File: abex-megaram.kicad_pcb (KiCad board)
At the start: 2 copper layers, 135.5 x 71.5 mm, 56 parts, among them P1 0877159106, P2 CONN_01X01, P3 CONN_01X01, P4 CONN_01X01, P5 CONN_01X01, P6 CONN_01X01, SW1 SW_DIP_x03, SW2 SW_Push, U1 74HC04, U14 STM32F407VGTx, U7 ISSI61WV5128BL, U8 ISSI61WV5128BL

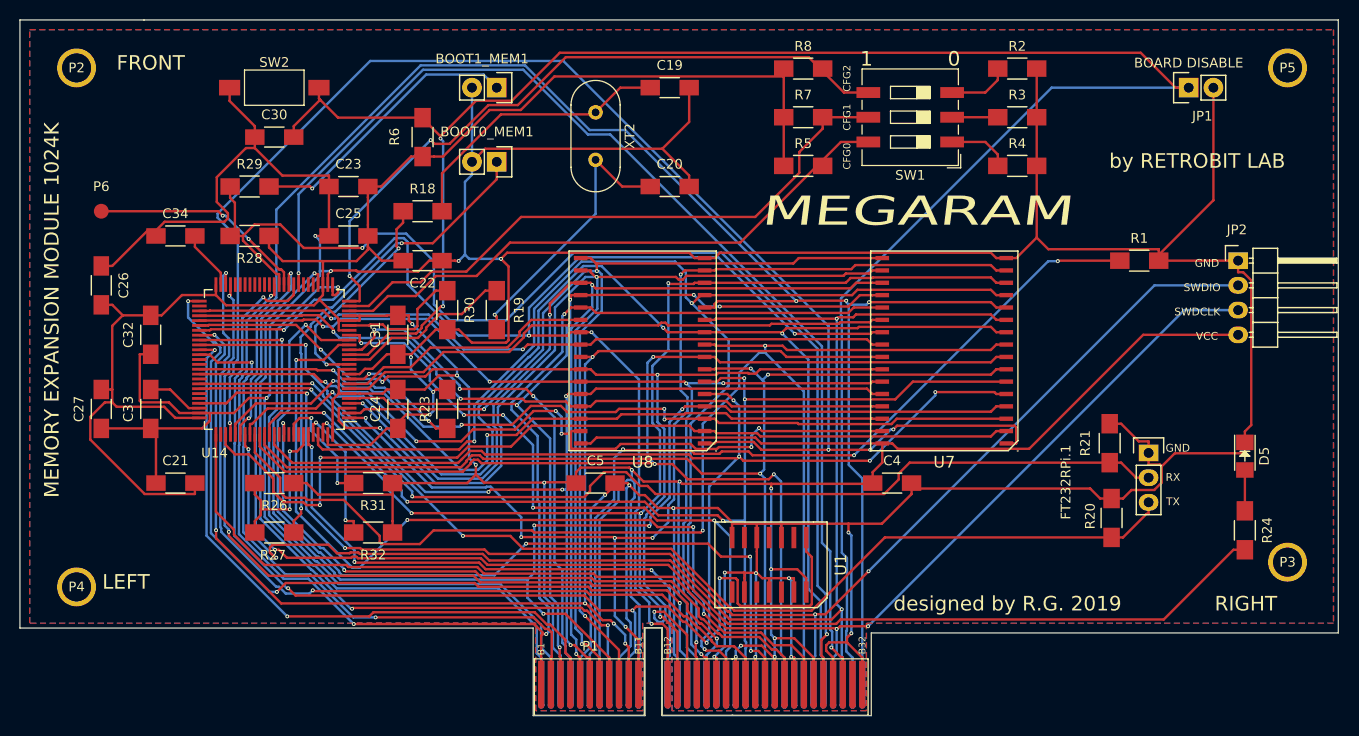
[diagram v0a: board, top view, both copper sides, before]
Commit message: New layout and design
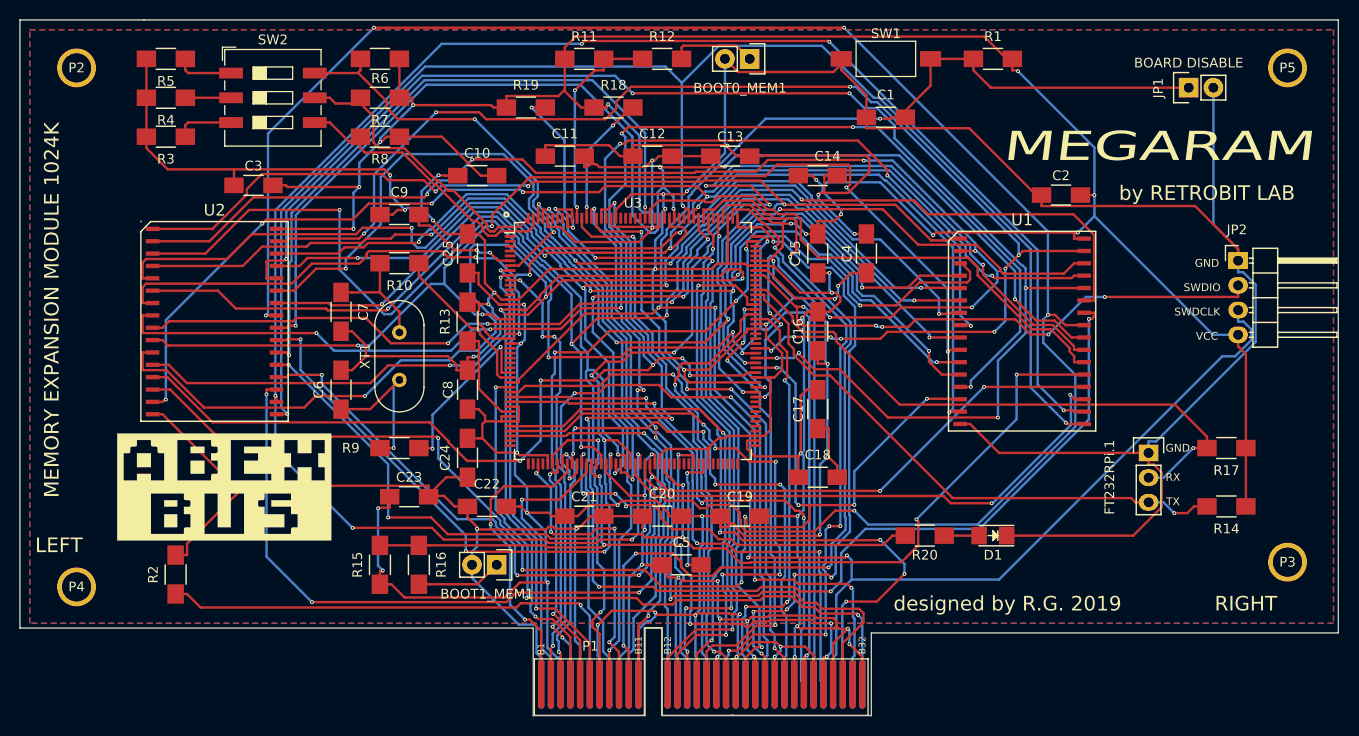
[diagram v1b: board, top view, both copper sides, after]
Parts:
- removed C26, C27, C30, C31: 100n, Capacitors_SMD:C_1206_HandSoldering
- removed C32: 1u, Capacitors_SMD:C_1206_HandSoldering
- removed C33, C34: 2.2u, Capacitors_SMD:C_1206_HandSoldering
- removed D5: LED.GREEN, LEDs:LED_1206
- removed P6: CONN_01X01, Measurement_Points:Measurement_Point_Round-SMD-Pad_Small
- removed R21, R26, R28: 10K, Resistors_SMD:R_1206_HandSoldering
- removed R23, R30: 0, Resistors_SMD:R_1206_HandSoldering
- removed R24: 220, Resistors_SMD:R_1206_HandSoldering
- removed R27, R29: 510, Resistors_SMD:R_1206_HandSoldering
- removed R31, R32: 4.7K, Resistors_SMD:R_1206_HandSoldering
- removed U14: STM32F407VGTx, Housings_QFP:TQFP-100_14x14mm_Pitch0.5mm
- removed U7, U8: ISSI61WV5128BL, RetroBitLab:SOP-32L-20.5x11.30-1.27mm
- removed XT2: 8Mhz, RetroBitLab:Crystal_HC49-4H_Vertical_3D
- added C1: 100n, Capacitors_SMD:C_1206_HandSoldering, F.Cu at (167.0, 64.0)
- added C10: 100n, Capacitors_SMD:C_1206_HandSoldering, F.Cu at (125.0, 70.0)
- added C11: 100n, Capacitors_SMD:C_1206_HandSoldering, F.Cu at (134.0, 68.0)
- added C12: 100n, Capacitors_SMD:C_1206_HandSoldering, F.Cu at (143.0, 68.0)
- added C13: 100n, Capacitors_SMD:C_1206_HandSoldering, F.Cu at (151.0, 68.0)
- added C14: 100n, Capacitors_SMD:C_1206_HandSoldering, F.Cu at (160.0, 70.0)
- added C15: 100n, Capacitors_SMD:C_1206_HandSoldering, F.Cu at (160.0, 78.0)
- added C16: 100n, Capacitors_SMD:C_1206_HandSoldering, F.Cu at (160.0, 86.0)
- added C17: 100n, Capacitors_SMD:C_1206_HandSoldering, F.Cu at (160.0, 94.0)
- added C18: 100n, Capacitors_SMD:C_1206_HandSoldering, F.Cu at (160.0, 101.0)
- added C2: 100n, Capacitors_SMD:C_1206_HandSoldering, F.Cu at (185.0, 72.0)
- added C3: 100n, Capacitors_SMD:C_1206_HandSoldering, F.Cu at (102.0, 71.0)
- added C6: 20p, Capacitors_SMD:C_1206_HandSoldering, F.Cu at (111.0, 92.0)
- added C7: 20p, Capacitors_SMD:C_1206_HandSoldering, F.Cu at (111.0, 84.0)
- added C8: 100n, Capacitors_SMD:C_1206_HandSoldering, F.Cu at (124.0, 92.0)
- added C9: 1u, Capacitors_SMD:C_1206_HandSoldering, F.Cu at (117.0, 74.0)
- added D1: LED.GREEN, LEDs:LED_1206, F.Cu at (178.0, 107.0)
- added G***: LOGO, RetroBitLab:ABEX_Logo_22mmx11mm_WB, F.Cu at (99.0, 102.0)
- added R10: 220, Resistors_SMD:R_1206_HandSoldering, F.Cu at (117.0, 79.0)
- added R11: 10K, Resistors_SMD:R_1206_HandSoldering, F.Cu at (136.0, 58.0)
- added R12: 510, Resistors_SMD:R_1206_HandSoldering, F.Cu at (144.0, 58.0)
- added R13: 0, Resistors_SMD:R_1206_HandSoldering, F.Cu at (124.0, 85.0)
- added R14: 10K, Resistors_SMD:R_1206_HandSoldering, F.Cu at (202.0, 104.0)
- added R15: 10K, Resistors_SMD:R_1206_HandSoldering, F.Cu at (115.0, 110.0)
- added R16: 510, Resistors_SMD:R_1206_HandSoldering, F.Cu at (119.0, 110.0)
- added R17: 10K, Resistors_SMD:R_1206_HandSoldering, F.Cu at (202.0, 98.0)
- added R9: 0, Resistors_SMD:R_1206_HandSoldering, F.Cu at (117.0, 98.0)
- added U2: ISSI61WV5128BL, RetroBitLab:SOP-32L-20.5x11.30-1.27mm, F.Cu at (98.0, 85.0)
- added U3: STM32F407IGTx, Housings_QFP:LQFP-176_24x24mm_Pitch0.5mm, F.Cu at (141.0, 87.0)
- added XT1: 8Mhz, RetroBitLab:Crystal_HC49-4H_Vertical_3D, F.Cu at (117.0, 91.0)
- C19, C20: value 20p -> 100n
- C4, C5: value 100n -> 2.2u
- R1: value 0 -> 100K
- R18: value 0 -> 4.7K
- R19: value 220 -> 4.7K
- R2: value 470 -> 0
- R20: value 10K -> 220
- R5: value 4.7K -> 470
- R6: value 100K -> 4.7K
- SW1: value SW_DIP_x03 -> SW_Push; footprint RetroBitLab:SW_DIP_SPSTx03_Slide_9.78x9.8mm_W8.61mm_P2.54mm -> RetroBitLab:SW_SPST_FSMSM_3D
- SW2: value SW_Push -> SW_DIP_x03; footprint RetroBitLab:SW_SPST_FSMSM_3D -> RetroBitLab:SW_DIP_SPSTx03_Slide_9.78x9.8mm_W8.61mm_P2.54mm
- U1: value 74HC04 -> ISSI61WV5128BL; footprint RetroBitLab:PSOP14-5x7.40-1.27 -> RetroBitLab:SOP-32L-20.5x11.30-1.27mm
- moved R2 100.9 mm to (94.0, 111.0), turned to 90 degrees
- moved R4 87.8 mm to (93.0, 62.0), turned to 180 degrees
- moved R3 87.5 mm to (93.0, 66.0), turned to 180 degrees
- moved R5 66.4 mm to (93.0, 58.0), turned to 180 degrees
- moved BOOT1_MEM1 49.0 mm to (127.0, 110.0)
- moved C19 44.6 mm to (152.0, 105.0), turned to 180 degrees
- moved R8 44.1 mm to (115.0, 66.0), turned to 180 degrees
- moved R7 43.5 mm to (115.0, 62.0), turned to 180 degrees
- moved C21 42.2 mm to (136.0, 105.0), turned to 180 degrees
- moved U1 35.4 mm to (181.0, 86.0), turned to 270 degrees
- moved C20 33.9 mm to (144.0, 105.0)
- moved C23 32.5 mm to (118.0, 103.0), turned to 180 degrees
- moved BOOT0_MEM1 28.1 mm to (153.0, 58.0)
- moved C22 26.1 mm to (126.0, 104.0), turned to 0 degrees
- moved R1 25.6 mm to (178.0, 58.0)
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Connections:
- C19 pad 1: Net-(C19-Pad1) -> GND
- C19 pad 2: GND -> VCC_3V3
- C20 pad 1: Net-(C20-Pad1) -> GND
- C20 pad 2: GND -> VCC_3V3
- C4 pad 1: VCC_3V3 -> GND
- C4 pad 2: GND -> VCAP_2_MEM
- C5 pad 1: VCC_3V3 -> GND
- C5 pad 2: GND -> VCAP_1_MEM
- R1 pad 1: mAUDIO -> SWDRST
- R1 pad 2: GND -> VCC_3V3
- R18 pad 1: Net-(R18-Pad1) -> VCC_3V3
- R18 pad 2: Net-(C19-Pad1) -> PB6
- R19 pad 1: Net-(R19-Pad1) -> VCC_3V3
- R19 pad 2: Net-(C20-Pad1) -> PB9
- R2 pad 1: Net-(R2-Pad1) -> mAUDIO
- R20 pad 1: GND -> Net-(D1-Pad2)
- R20 pad 2: UART_TX -> LEDGRN_MEM
- R5 pad 1: VCC_3V3 -> Net-(R5-Pad1)
- R5 pad 2: mCONF0 -> GND
- R6 pad 1: SWDRST -> VCC_3V3
- R6 pad 2: VCC_3V3 -> mCONF0
- SW1 pad 1: Net-(R4-Pad1) -> GND
- SW1 pad 2: Net-(R3-Pad1) -> SWDRST
- SW2 pad 1: GND -> Net-(R5-Pad1)
- SW2 pad 2: SWDRST -> Net-(R4-Pad1)
- U1 pad 1: mR/~W -> FSMC_A17
- U1 pad 10: (no net) -> FSMC_A2
- U1 pad 11: GND -> FSMC_A1
- U1 pad 12: (no net) -> FSMC_A0
- U1 pad 13: GND -> FSMC_D0
- U1 pad 14: VCC_3V3 -> FSMC_D1
- U1 pad 2: (no net) -> FSMC_A16
- U1 pad 3: GND -> FSMC_A14
- U1 pad 4: (no net) -> FSMC_A12
- U1 pad 5: GND -> FSMC_A7
- U1 pad 6: (no net) -> FSMC_A6
- U1 pad 7: GND -> FSMC_A5
- U1 pad 8: (no net) -> FSMC_A4
- U1 pad 9: GND -> FSMC_A3
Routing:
- net FSMC_A11: track 0.00 -> 194.5 mm, vias 0 -> 5
- net FSMC_D4: track 0.00 -> 190.5 mm, vias 0 -> 7
- net FSMC_D0: track 0.00 -> 164.0 mm, vias 0 -> 8
- net FSMC_A10: track 0.00 -> 155.6 mm, vias 0 -> 9
- net FSMC_A9: track 0.00 -> 154.4 mm, vias 0 -> 5
- net mB3: track 153.4 -> 0.00 mm, vias 4 -> 0
- net FSMC_D3: track 0.00 -> 152.0 mm, vias 0 -> 3
- net FSMC_A13: track 0.00 -> 150.9 mm, vias 0 -> 7
- net FSMC_A16: track 0.00 -> 144.5 mm, vias 0 -> 9
- net FSMC_A8: track 0.00 -> 141.0 mm, vias 0 -> 5
- net FSMC_A15: track 0.00 -> 136.1 mm, vias 0 -> 10
- net FSMC_NOE: track 0.00 -> 131.4 mm, vias 0 -> 5
- net FSMC_A14: track 0.00 -> 130.5 mm, vias 0 -> 5
- net FSMC_D1: track 0.00 -> 128.8 mm, vias 0 -> 8
- net FSMC_A7: track 0.00 -> 128.6 mm, vias 0 -> 5
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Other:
- board text removed: "0"
- board text removed: "1"
- board text removed: "CFG0"
- board text removed: "CFG1"
- board text removed: "CFG2"
- board text removed: "FRONT"
